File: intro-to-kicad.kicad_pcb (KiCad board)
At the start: 2 copper layers, 100 x 60 mm, 20 parts, among them J1 Conn_01x01_Pin, J2 Conn_01x02_Pin, J3 Conn_01x02_Pin, U1 NE555P

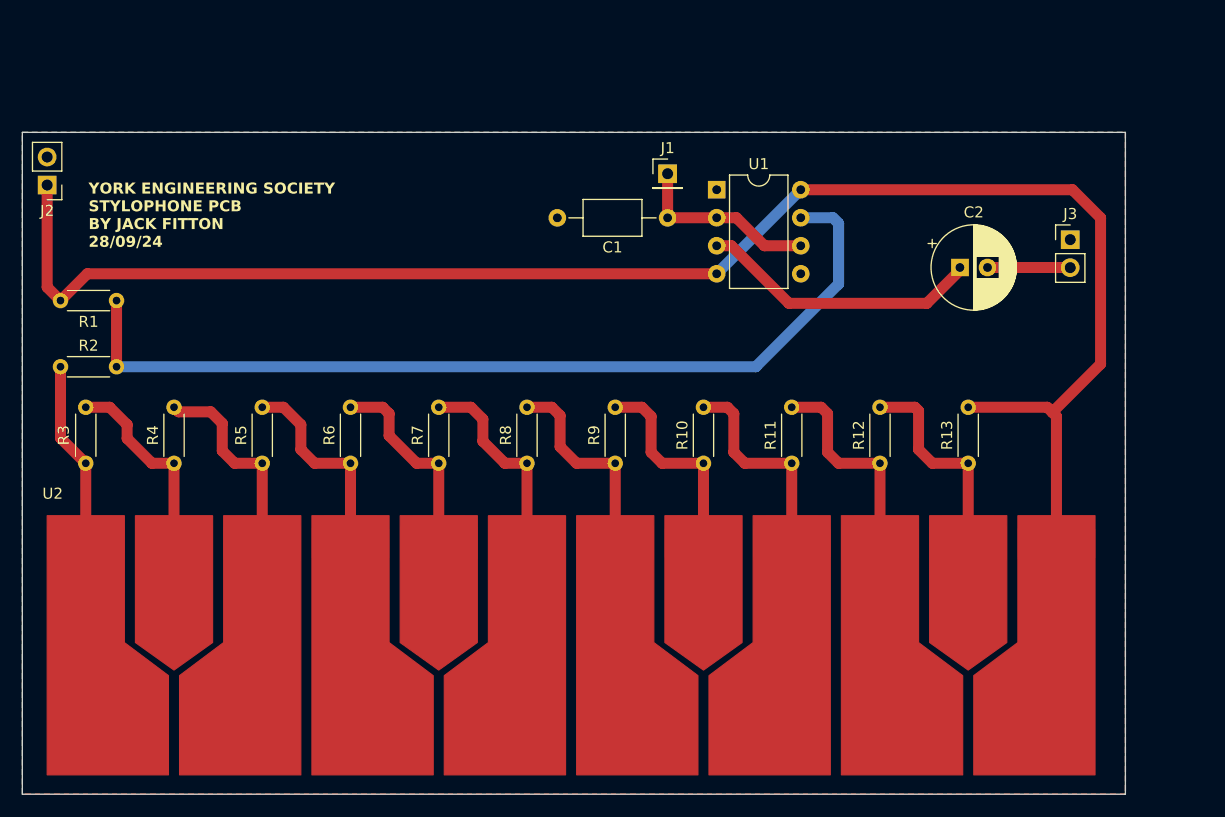
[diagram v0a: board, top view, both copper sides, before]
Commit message: finalised project
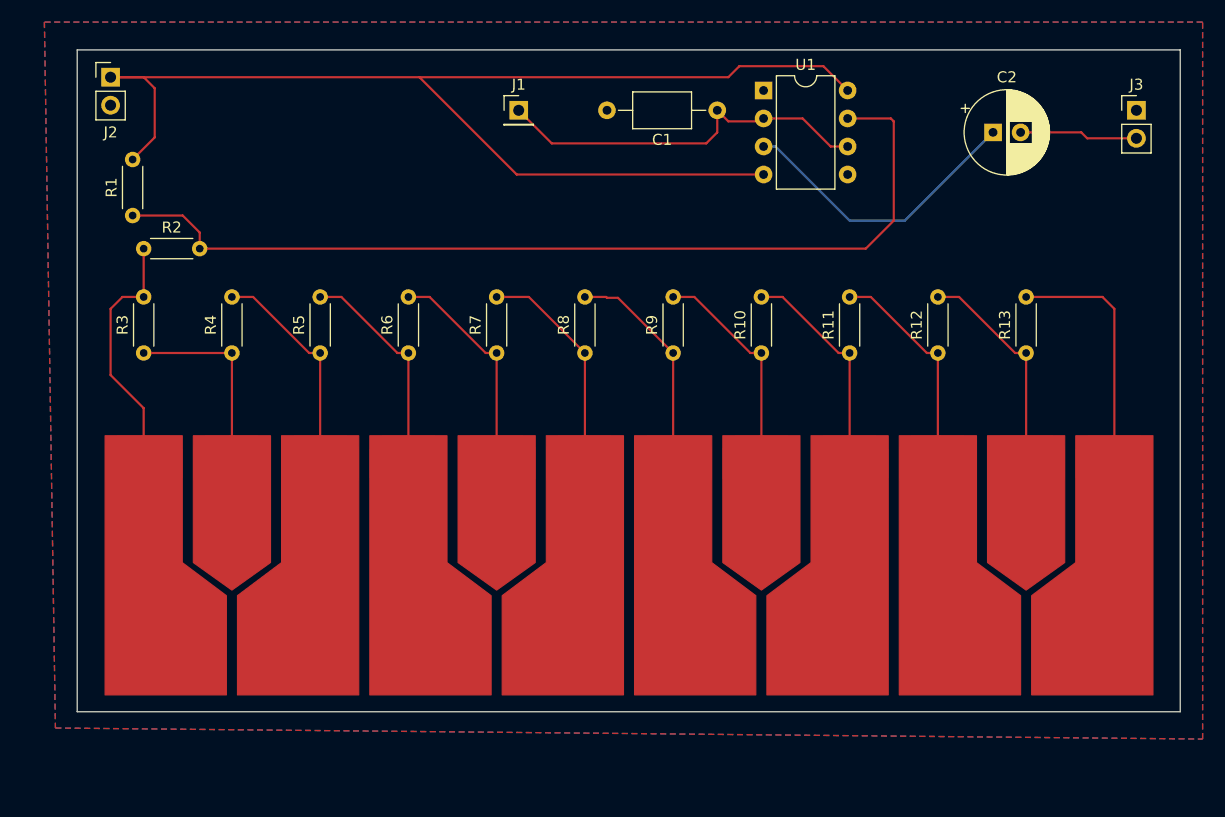
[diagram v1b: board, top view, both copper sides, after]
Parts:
- R10: value 626 -> 30K
- R11: value 650 -> 30K
- R12: value 690 -> 30K
- R13: value 730 -> 30K
- R2: value 1876 -> 30K
- R3: value 411 -> 30K
- R4: value 438 -> 30K
- R5: value 456 -> 30k
- R6: value 482 -> 30k
- R7: value 520 -> 30K
- R8: value 546 -> 30K
- R9: value 570 -> 30K
- moved J1 14.7 mm to (145.0, 68.0)
- moved J3 13.2 mm to (201.0, 68.0)
- moved R2 13.1 mm to (111.0, 80.5)
- moved C2 12.6 mm to (188.0, 70.0)
- moved J2 11.3 mm to (108.0, 65.0), turned to 0 degrees
- moved R10 11.3 mm to (167.0, 90.0)
- moved R11 11.3 mm to (175.0, 90.0)
- moved R12 11.3 mm to (183.0, 90.0)
- moved R13 11.3 mm to (191.0, 90.0)
- moved R4 11.3 mm to (119.0, 90.0)
- moved R5 11.3 mm to (127.0, 90.0)
- moved R6 11.3 mm to (135.0, 90.0)
- moved R7 11.3 mm to (143.0, 90.0)
- moved R8 11.3 mm to (151.0, 90.0)
- moved R9 11.3 mm to (159.0, 90.0)
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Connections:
- R13 pad 2: +9V -> /KEY_12
- U2 pad 12: +9V -> /KEY_12
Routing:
- net +9V: track 149.8 -> 114.7 mm
- net /KEY_12: track 0.00 -> 22.4 mm
- net STYLUS: track 17.1 -> 35.1 mm
- net /KEY_1: track 16.9 -> 23.1 mm
- net /SPKR+: track 7.51 -> 10.7 mm
- net /555_DIS: track 83.7 -> 85.4 mm
- net /KEY_6: track 18.5 -> 20.1 mm
- net /KEY_5: track 18.5 -> 20.1 mm
- net /KEY_4: track 18.7 -> 20.1 mm
- net /KEY_3: track 18.8 -> 20.1 mm
- net /555_Q: track 25.7 -> 26.9 mm
- net /KEY_7: track 19.0 -> 20.1 mm
- net /KEY_8: track 19.3 -> 20.1 mm
- net /KEY_9: track 19.4 -> 20.1 mm
- net /KEY_11: track 19.4 -> 20.1 mm
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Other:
- board text removed: "YORK ENGINEERING SOCIETY STYLOPHONE PCB BY JACK FITTON 28/09/24"
